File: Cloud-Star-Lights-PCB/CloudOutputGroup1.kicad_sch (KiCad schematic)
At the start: 3 parts, among them J33 Conn_01x04

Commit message: Starting routing
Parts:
- J33: footprint (none) -> Connector_PinHeader_2.54mm:PinHeader_1x04_P2.54mm_Vertical
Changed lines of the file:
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@@
       (effects (font (size 1.27 1.27)) (justify left))
     )
-    (property "Footprint" "" (at 134.62 40.64 0)
+    (property "Footprint" "Connector_PinHeader_2.54mm:PinHeader_1x04_P2.54mm_Vertical" (at 134.62 40.64 0)
       (effects (font (size 1.27 1.27)) hide)
     )
@@
       (effects (font (size 1.27 1.27)) (justify left))
     )
-    (property "Footprint" "" (at 134.62 68.58 0)
+    (property "Footprint" "Connector_PinHeader_2.54mm:PinHeader_1x04_P2.54mm_Vertical" (at 134.62 68.58 0)
       (effects (font (size 1.27 1.27)) hide)
     )
@@
       (effects (font (size 1.27 1.27)) (justify left))
     )
-    (property "Footprint" "" (at 134.7586 54.6962 0)
+    (property "Footprint" "Connector_PinHeader_2.54mm:PinHeader_1x04_P2.54mm_Vertical" (at 134.7586 54.6962 0)
       (effects (font (size 1.27 1.27)) hide)
     )

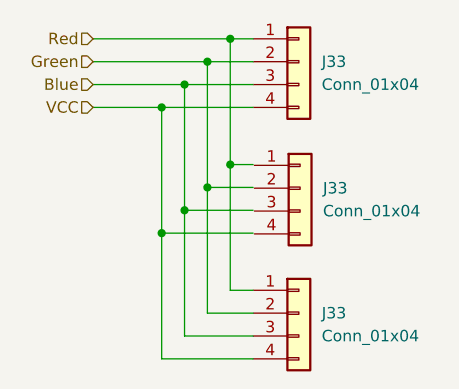
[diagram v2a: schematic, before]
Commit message: Unrouted board
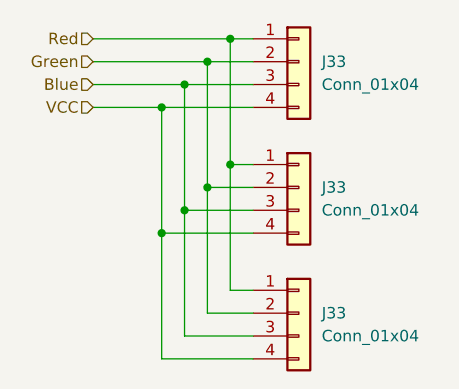
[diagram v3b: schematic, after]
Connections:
- net Blue: now also J33.3 (Pin_3)
- net Green: now also J33.2 (Pin_2)
- net Red: now also J33.1 (Pin_1)
- net VCC: now also J33.4 (Pin_4)
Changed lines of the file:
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@@
     )
   )
-  (symbol (lib_id "Connector_Generic:Conn_01x04") (at 134.7586 54.6962 0) (unit 1)
+  (symbol (lib_id "Connector_Generic:Conn_01x04") (at 134.62 54.61 0) (unit 1)
     (in_bom yes) (on_board yes) (dnp no) (fields_autoplaced)
-    (property "Reference" "J33" (at 137.2986 54.6962 0)
+    (property "Reference" "J33" (at 137.16 54.61 0)
       (effects (font (size 1.27 1.27)) (justify left))
     )
-    (property "Value" "Conn_01x04" (at 137.2986 57.2362 0)
+    (property "Value" "Conn_01x04" (at 137.16 57.15 0)
       (effects (font (size 1.27 1.27)) (justify left))
     )
-    (property "Footprint" "Connector_PinHeader_2.54mm:PinHeader_1x04_P2.54mm_Vertical" (at 134.7586 54.6962 0)
+    (property "Footprint" "Connector_PinHeader_2.54mm:PinHeader_1x04_P2.54mm_Vertical" (at 134.62 54.61 0)
       (effects (font (size 1.27 1.27)) hide)
     )
-    (property "Datasheet" "~" (at 134.7586 54.6962 0)
+    (property "Datasheet" "~" (at 134.62 54.61 0)
       (effects (font (size 1.27 1.27)) hide)
     )
